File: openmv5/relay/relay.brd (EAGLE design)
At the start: 35.6 x 26.7 mm, 77 parts, among them IC1 TPS613222ADBVR, IC2 AP64060WU-7, IC3 LM321LVIDCKR, IC4 74LVC1G07GW,125, J1 OPENMV5-TOP, J2 1771088, K1 IMC03TS, K2 IMC03TS, Q1 SSM3J356R,LF, Q2 2N7002KW_R1_00001, Q3 2N7002KW_R1_00001, U1 74LVC1G17SE-7

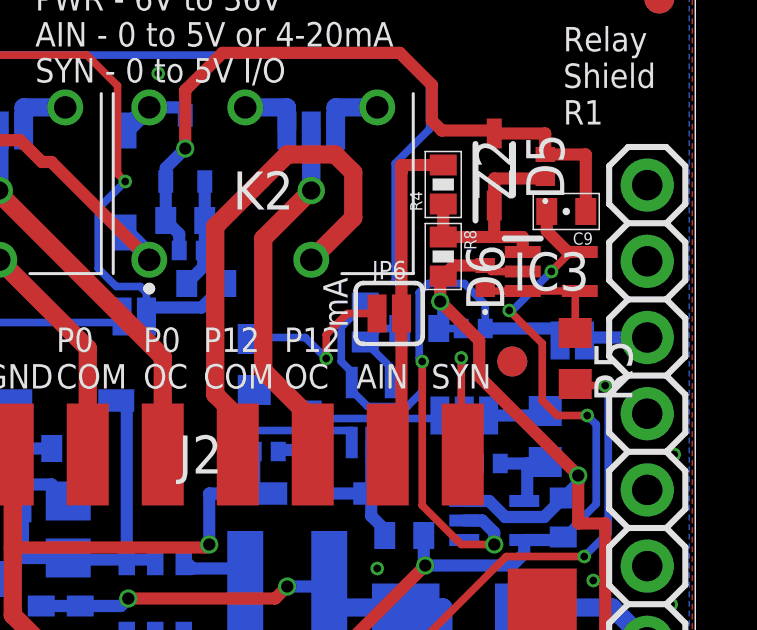
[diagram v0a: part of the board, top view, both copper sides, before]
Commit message: Fix wire stubs
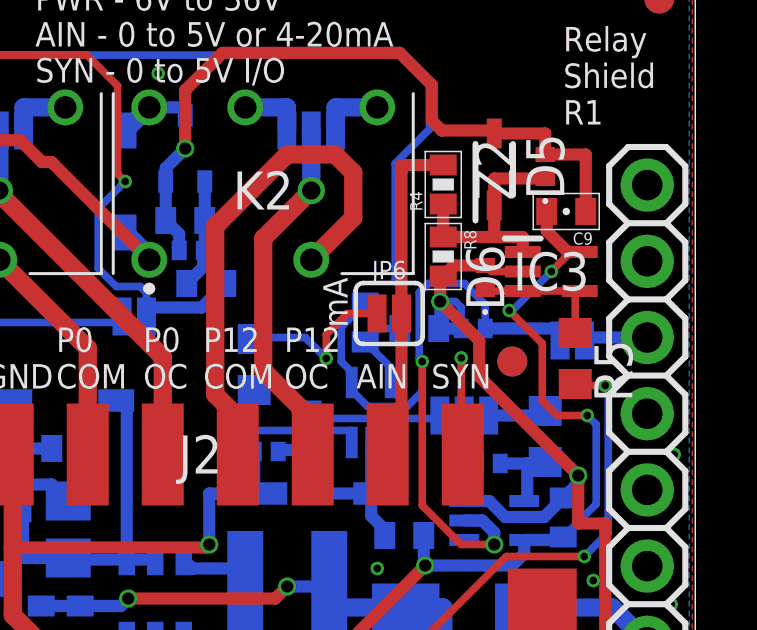
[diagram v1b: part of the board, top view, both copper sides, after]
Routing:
- net GND: track 159.5 -> 160.8 mm
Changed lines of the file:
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@@
 <via x="6.6" y="11.3" extent="1-16" drill="0.4064"/>
 <via x="6.8" y="7.1" extent="1-16" drill="0.254"/>
-<wire x1="27.1" y1="15.5" x2="27.2" y2="15.4" width="0.4064" layer="16"/>
-<wire x1="27.2" y1="15.4" x2="27.2" y2="14.6" width="0.4064" layer="16"/>
-<wire x1="27.8" y1="14.7" x2="27.8" y2="14.6" width="0.4064" layer="16"/>
 <contactref element="D10" pad="2"/>
 <contactref element="R14" pad="1"/>
@@
 <contactref element="R15" pad="1"/>
 <contactref element="Q3" pad="2"/>
-<wire x1="27.1" y1="15.5" x2="28.4" y2="14.2" width="0.4064" layer="1"/>
 <wire x1="28.4" y1="13" x2="31.7" y2="9.7" width="0.4064" layer="1"/>
 <wire x1="28.4" y1="14.2" x2="28.4" y2="13" width="0.4064" layer="1"/>
@@
 <wire x1="30.5666" y1="8.3166" x2="29.266425" y2="8.3166" width="0.4064" layer="16"/>
 <wire x1="27.9" y1="8.85" x2="28.733025" y2="8.85" width="0.4064" layer="16"/>
-<wire x1="27.8" y1="14.6" x2="27.05" y2="14.6" width="0.254" layer="16"/>
 <wire x1="7.55" y1="19.5" x2="7.55" y2="18.2" width="0.4064" layer="16"/>
 <wire x1="17.95" y1="19.5" x2="17.95" y2="18.2" width="0.4064" layer="16"/>
@@
 <via x="34.9" y="10.4" extent="1-16" drill="0.254"/>
 <via x="34.8" y="5.4" extent="1-16" drill="0.254"/>
+<wire x1="27.1" y1="15.5" x2="27.1" y2="14.65" width="0.4064" layer="16"/>
+<wire x1="27.1" y1="14.65" x2="27.05" y2="14.6" width="0.4064" layer="16"/>
+<wire x1="27.8" y1="14.6" x2="27.15" y2="14.6" width="0.4064" layer="16"/>
+<wire x1="27.15" y1="14.6" x2="27.1" y2="14.65" width="0.4064" layer="16"/>
+<wire x1="27.1" y1="15.5" x2="28.4" y2="14.2" width="0.4064" layer="1"/>
+<wire x1="27.8" y1="14.6" x2="27.8" y2="15.3" width="0.254" layer="16"/>
+<wire x1="27.6" y1="15.5" x2="27.1" y2="15.5" width="0.254" layer="16"/>
+<wire x1="27.8" y1="15.3" x2="27.6" y2="15.5" width="0.254" layer="16"/>
 </signal>
 <signal name="N$69">
